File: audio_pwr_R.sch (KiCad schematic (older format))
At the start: 40 parts, among them Q201 BC546, Q202 BC546, Q203 BC546, Q204 BD140, Q205 BC546, Q206 BD139, Q207 BD140, Q208 MJL21193, Q209 MJL21194

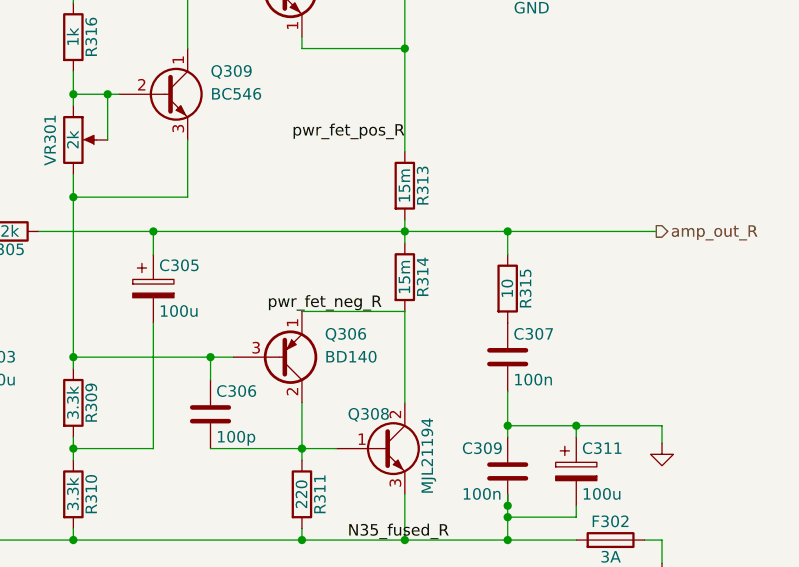
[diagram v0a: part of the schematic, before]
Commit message: 23JAN2020 daily commit.
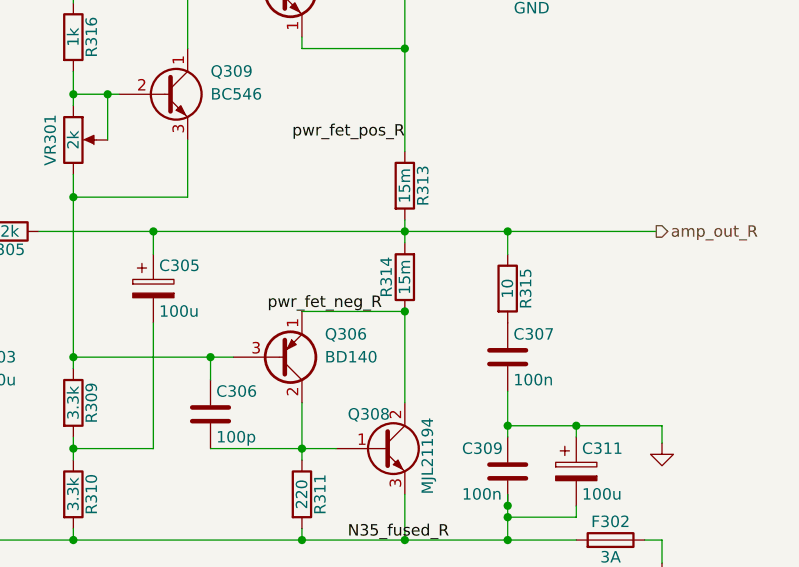
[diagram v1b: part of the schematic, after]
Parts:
- R214, R215: footprint Resistor_THT:R_Axial_Power_L25.0mm_W9.0mm_P30.48mm -> Resistor_THT:R_Axial_Power_L25.0mm_W9.0mm_P10.16mm_Vertical
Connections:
- net amp_out_R: now also R215.2; no longer R215.1
- net pwr_fet_neg_R: now also R215.1; no longer R215.2
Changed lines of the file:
@@
 F 0 "R314" V 6980 3850 50  0000 C CNN
 F 1 "15m" V 6900 3850 50  0000 C CNN
-F 2 "Resistor_THT:R_Axial_Power_L25.0mm_W9.0mm_P30.48mm" V 6830 3850 50  0001 C CNN
+F 2 "Resistor_THT:R_Axial_Power_L25.0mm_W9.0mm_P10.16mm_Vertical" V 6830 3850 50  0001 C CNN
 F 3 "" H 6900 3850 50  0001 C CNN
 	1    6900 3850
-	1    0    0    -1
+	-1   0    0    1
 $EndComp
 $Comp
@@
 F 0 "R313" V 6980 3450 50  0000 C CNN
 F 1 "15m" V 6900 3450 50  0000 C CNN
-F 2 "Resistor_THT:R_Axial_Power_L25.0mm_W9.0mm_P30.48mm" V 6830 3450 50  0001 C CNN
+F 2 "Resistor_THT:R_Axial_Power_L25.0mm_W9.0mm_P10.16mm_Vertical" V 6830 3450 50  0001 C CNN
 F 3 "" H 6900 3450 50  0001 C CNN
 	1    6900 3450
@@
 	8025 4500 7650 4500
 Connection ~ 7650 4500
+Connection ~ 6900 4000
 $EndSCHEMATC
